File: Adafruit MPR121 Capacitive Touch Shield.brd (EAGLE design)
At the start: 68.6 x 53.3 mm, 53 parts, among them Q1 BSS138, Q2 BSS138, SW2 SPST_TACT-EVQQ2, U2 MPR121, U4 MIC5225-3.3

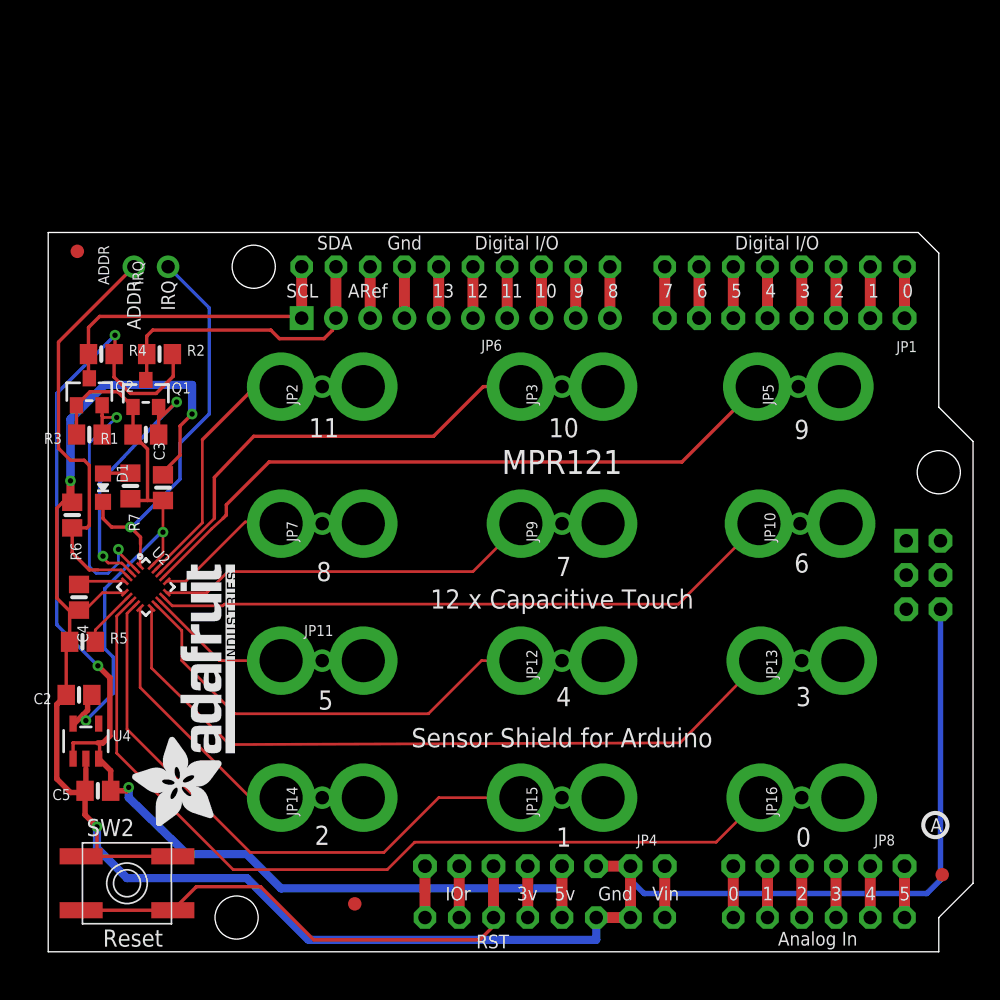
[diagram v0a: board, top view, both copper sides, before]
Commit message: Add updated board files.
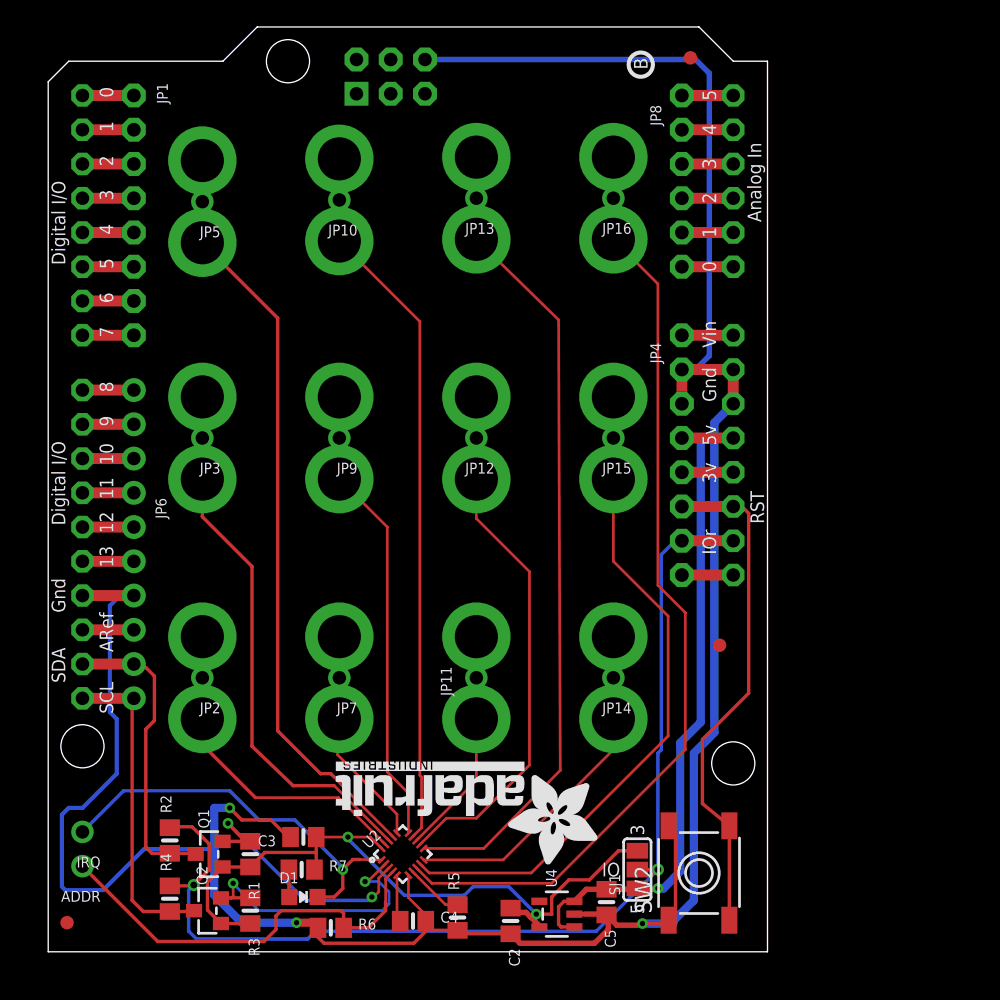
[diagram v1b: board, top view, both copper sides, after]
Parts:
- added PLABEL0: (no value), pinguin:PLABEL0
- added PLABEL1: (no value), pinguin:PLABEL1
- added PLABEL10: (no value), pinguin:PLABEL10
- added PLABEL11: (no value), pinguin:PLABEL11
- added PLABEL12: (no value), pinguin:PLABEL12
- added PLABEL13: (no value), pinguin:PLABEL13
- added PLABEL14: (no value), pinguin:PLABEL14
- added PLABEL15: (no value), pinguin:PLABEL15
- added PLABEL16: (no value), pinguin:PLABEL16
- added PLABEL17: (no value), pinguin:PLABEL17
- added PLABEL2: (no value), pinguin:PLABEL2
- added PLABEL3: (no value), pinguin:PLABEL3
- added PLABEL4: (no value), pinguin:PLABEL4
- added PLABEL5: (no value), pinguin:PLABEL5
- added PLABEL6: (no value), pinguin:PLABEL6
- added PLABEL7: (no value), pinguin:PLABEL7
- added PLABEL8: (no value), pinguin:PLABEL8
- added PLABEL9: (no value), pinguin:PLABEL9
- added SJ1: (no value), microbuilder:SOLDERJUMPER_2WAY_OPEN_NOPASTE
- AL1, AL10, AL11, AL12, AL2, AL3, AL4, AL5, AL6, AL7, AL8, AL9: device microbuilder:ALLIGATORCLIP -> adafruit_electromech:ALLIGATORCLIP
- FID1, FID2, FID3: value FIDUCIAL"" -> FIDUCIAL_1MM
- SW2: value SPST_TACT-EVQQ2 -> 6mm tact; device adafruit:EVQ-Q2 -> adafruit_electromech:6MMX6MM_TACTILE_SMT
- U$41: value ARDUINO_R3_ICSP -> ARDUINO_R3_ICSP_NODIM; device adafruit:ARDUINOR3_ICSP -> adafruit:ARDUINOR3_ICSP_NODIM
- U2: device microbuilder:QFN20_3MM_NOTHERMAL -> adafruit_sensor:QFN20_3MM_NOTHERMAL
- U4: value MIC5225-3.3 -> AP2127K-3.3; device microbuilder:SOT23-5 -> adafruit_power:SOT23-5
- moved FID2 63.4 mm to (47.6, 66.3), turned to 90 degrees
- moved U$8 60.5 mm to (43.9, 65.8), turned to 90 degrees
- moved U$41 53.3 mm to (53.3, 0.00), turned to 90 degrees
- moved JP8 51.8 mm to (47.0, 57.1), turned to 270 degrees
- moved FID3 49.8 mm to (1.40, 2.16), turned to 90 degrees
- moved JP1 48.9 mm to (6.35, 54.6), turned to 90 degrees
- moved AL1 46.6 mm to (41.9, 55.9), turned to 180 degrees
- moved JP16 46.6 mm to (41.9, 55.9), turned to 180 degrees
- moved AL10 46.3 mm to (11.4, 55.6), turned to 180 degrees
- moved JP5 46.3 mm to (11.4, 55.6), turned to 180 degrees
- moved ADDR 44.6 mm to (2.54, 6.35), turned to 180 degrees
- moved SW2 42.4 mm to (48.3, 5.84), turned to 90 degrees
- moved IRQ 42.4 mm to (2.54, 8.89), turned to 180 degrees
- moved AL4 41.9 mm to (31.8, 55.9), turned to 180 degrees
- moved JP13 41.9 mm to (31.8, 55.9), turned to 180 degrees
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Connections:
- removed net IORESET: JP4.7, U$41.IOREF
- new net VCCIO: JP4.7, R2.2, R4.2, SJ1.2, U$41.IOREF
- net +5V: now also SJ1.1; no longer R2.2, R4.2
- net 3.3V: now also SJ1.3
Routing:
- net VCCIO: track 0.00 -> 81.3 mm, vias 0 -> 2
- net +5V: track 95.1 -> 53.0 mm, vias 3 -> 1
- net GND: track 169.5 -> 204.5 mm
- net 3.3V: track 42.6 -> 52.8 mm
- net IORESET: track 3.81 -> 0.00 mm
- net ELEC0: track 71.4 -> 70.7 mm
- net SDA_3V: track 20.7 -> 20.0 mm
- net ELEC1: track 50.3 -> 49.7 mm
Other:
- board size 68.6 x 53.3 mm -> 53.3 x 68.6 mm
- board text added: "IO"
